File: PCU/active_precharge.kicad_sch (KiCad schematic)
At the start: 32 parts, among them IC32 LM5060MMX_NOPB, Q21 BC846B, Q22 DMP6023LFG-7, Q23 NTMFS5H600NLT1G, Q24 NTMFS5H600NLT1G, Q25 NTMFS5H600NLT1G, Q26 NTMFS5H600NLT1G, Q27 BC846B

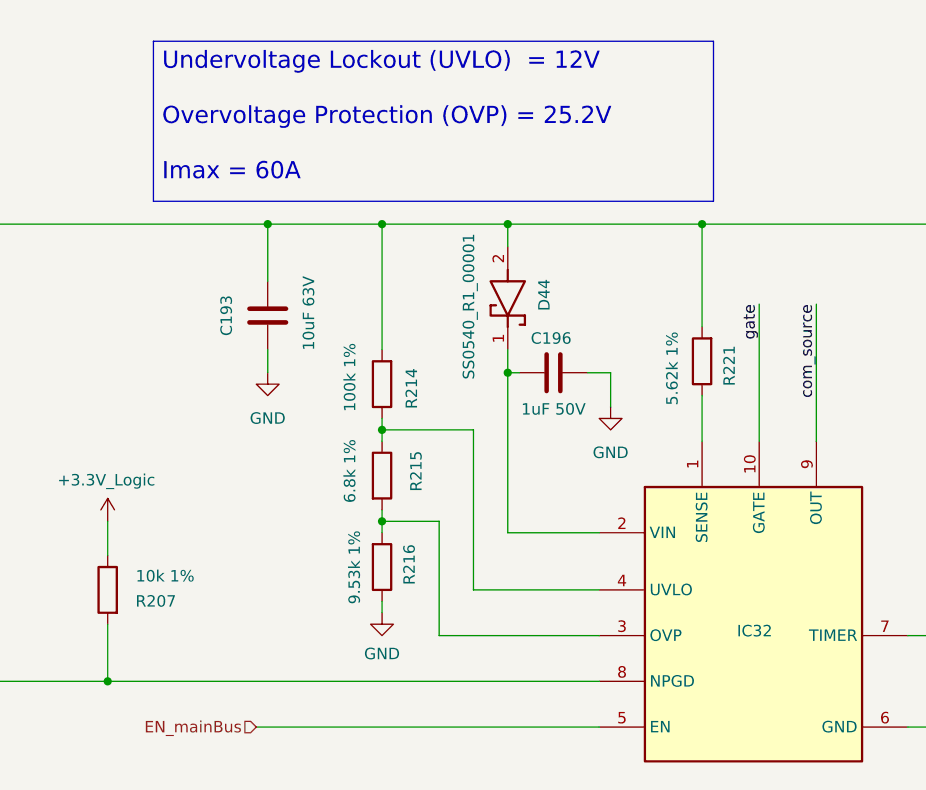
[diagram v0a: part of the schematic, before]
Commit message: PCB Design started
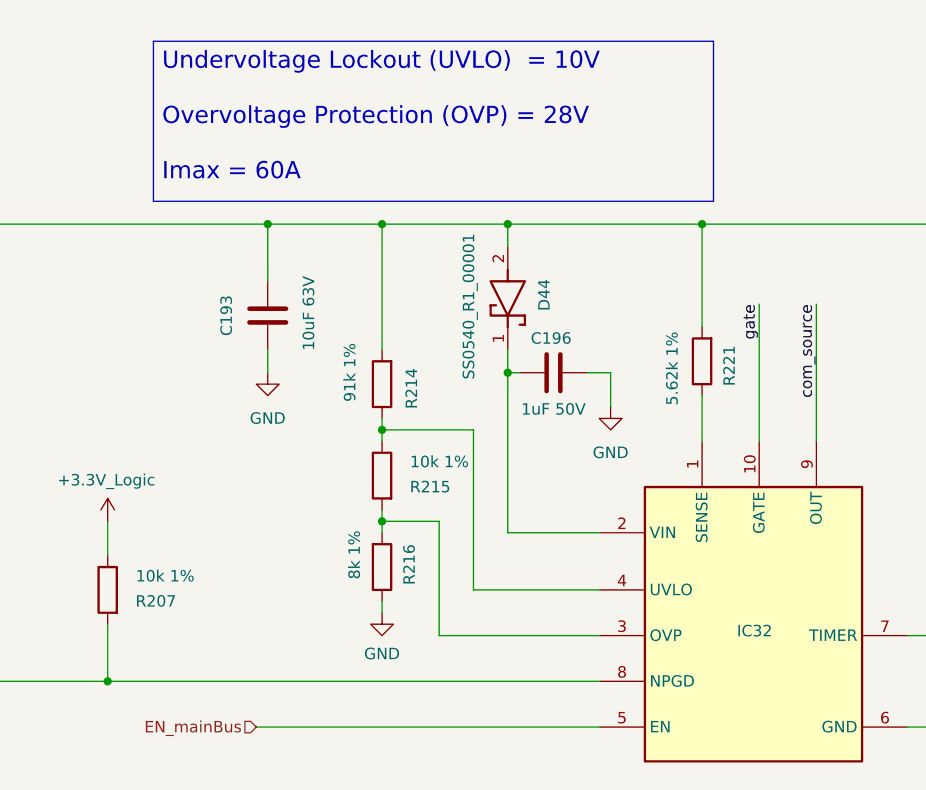
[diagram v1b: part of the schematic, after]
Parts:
- R214: value 100k 1% -> 91k 1%; Manufacturer_Part_Number AT0603FRE07100KL -> RT0603BRD0791KL
- R215: value 6.8k 1% -> 10k 1%; Manufacturer_Part_Number AC0603FR-076K8L -> AF0603FR-0710KL
- R216: value 9.53k 1% -> 8k 1%; Manufacturer_Part_Number AF0603FR-079K53L -> RT0603BRE078KL
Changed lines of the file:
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@@
 		)
 	)
-	(text_box "Undervoltage Lockout (UVLO)  = 12V\n\nOvervoltage Protection (OVP) = 25.2V\n\nImax = 60A"
+	(text_box "Undervoltage Lockout (UVLO)  = 10V\n\nOvervoltage Protection (OVP) = 28V\n\nImax = 60A"
 		(exclude_from_sim no)
 		(at 53.34 17.78 0)
@@
 	(symbol
 		(lib_id "Device:R")
+		(at 78.74 66.04 0)
+		(mirror y)
+		(unit 1)
+		(exclude_from_sim no)
+		(in_bom yes)
+		(on_board yes)
+		(dnp no)
+		(property "Reference" "R215"
+			(at 86.36 67.31 0)
+			(effects
+				(font
+					(size 1.27 1.27)
+				)
+				(justify left)
+			)
+		)
+		(property "Value" "10k 1%"
+			(at 88.392 64.516 0)
+			(effects
+				(font
+					(size 1.27 1.27)
+				)
+				(justify left)
+			)
+		)
+		(property "Footprint" "Resistor_SMD:R_0603_1608Metric"
+			(at 80.518 66.04 90)
+			(effects
+				(font
+					(size 1.27 1.27)
+				)
+				(hide yes)
+			)
+		)
+		(property "Datasheet" "~"
+			(at 78.74 66.04 0)
+			(effects
+				(font
+					(size 1.27 1.27)
+				)
+				(hide yes)
+			)
+		)
+		(property "Description" "Resistor"
+			(at 78.74 66.04 0)
+			(effects
+				(font
+					(size 1.27 1.27)
+				)
+				(hide yes)
+			)
+		)
+		(property "Manufacturer_Name" "YAGEO"
+			(at 78.74 66.04 0)
+			(effects
+				(font
+					(size 1.27 1.27)
+				)
+				(hide yes)
+			)
+		)
+		(property "Manufacturer_Part_Number" "AF0603FR-0710KL"
+			(at 78.74 66.04 0)
+			(effects
+				(font
+					(size 1.27 1.27)
+				)
+				(hide yes)
+			)
+		)
+		(property "Packaging" "0603 (608mm)"
+			(at 78.74 66.04 0)
+			(effects
+				(font
+					(size 1.27 1.27)
+				)
+				(hide yes)
+			)
+		)
+		(pin "1"
+		)
+		(pin "2"
+		)
+		(instances
+			(project "PCU"
+				(path "/c5277b98-916c-45ac-b199-6b9ee16008ba/0aad7a0a-408b-4596-959e-c6df745f73d1"
+					(reference "R215")
+					(unit 1)
+				)
+			)
+		)
+	)
+	(symbol
+		(lib_id "Device:R")
 		(at 168.91 120.65 90)
 		(mirror x)
@@
 	(symbol
 		(lib_id "Device:R")
-		(at 78.74 66.04 0)
-		(unit 1)
-		(exclude_from_sim no)
-		(in_bom yes)
-		(on_board yes)
-		(dnp no)
-		(property "Reference" "R215"
-			(at 82.55 67.818 90)
-			(effects
-				(font
-					(size 1.27 1.27)
-				)
-				(justify left)
-			)
-		)
-		(property "Value" "6.8k 1%"
-			(at 75.184 69.088 90)
-			(effects
-				(font
-					(size 1.27 1.27)
-				)
-				(justify left)
-			)
-		)
-		(property "Footprint" "Resistor_SMD:R_0603_1608Metric"
-			(at 76.962 66.04 90)
-			(effects
-				(font
-					(size 1.27 1.27)
-				)
-				(hide yes)
-			)
-		)
-		(property "Datasheet" "~"
-			(at 78.74 66.04 0)
-			(effects
-				(font
-					(size 1.27 1.27)
-				)
-				(hide yes)
-			)
-		)
-		(property "Description" "Resistor"
-			(at 78.74 66.04 0)
-			(effects
-				(font
-					(size 1.27 1.27)
-				)
-				(hide yes)
-			)
-		)
-		(property "Manufacturer_Name" "YAGEO"
-			(at 78.74 66.04 0)
-			(effects
-				(font
-					(size 1.27 1.27)
-				)
-				(hide yes)
-			)
-		)
-		(property "Manufacturer_Part_Number" "AC0603FR-076K8L"
-			(at 78.74 66.04 0)
-			(effects
-				(font
-					(size 1.27 1.27)
-				)
-				(hide yes)
-			)
-		)
-		(property "Packaging" "0603 (608mm)"
-			(at 78.74 66.04 0)
-			(effects
-				(font
-					(size 1.27 1.27)
-				)
-				(hide yes)
-			)
-		)
-		(pin "1"
-		)
-		(pin "2"
-		)
-		(instances
-			(project "PCU"
-				(path "/c5277b98-916c-45ac-b199-6b9ee16008ba/0aad7a0a-408b-4596-959e-c6df745f73d1"
-					(reference "R215")
-					(unit 1)
-				)
-			)
-		)
-	)
-	(symbol
-		(lib_id "Device:R")
 		(at 99.06 133.35 180)
 		(unit 1)
@@
 			)
 		)
-		(property "Value" "100k 1%"
+		(property "Value" "91k 1%"
 			(at 75.184 51.308 90)
 			(effects
@@
 			)
 		)
-		(property "Manufacturer_Part_Number" "AT0603FRE07100KL"
+		(property "Manufacturer_Part_Number" "RT0603BRD0791KL"
 			(at 78.74 55.88 0)
 			(effects
@@
 			)
 		)
-		(property "Value" "9.53k 1%"
+		(property "Value" "8k 1%"
 			(at 75.692 72.136 90)
 			(effects
@@
 			)
 		)
-		(property "Manufacturer_Part_Number" "AF0603FR-079K53L"
+		(property "Manufacturer_Part_Number" "RT0603BRE078KL"
 			(at 78.74 76.2 0)
 			(effects
